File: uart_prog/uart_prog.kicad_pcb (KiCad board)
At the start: 2 copper layers, 22 parts, among them J1 USB_B_Micro, J2 Conn_01x06, Q1 MBT3904DW1, SW1 SW_SPDT, U1 FT231XQ

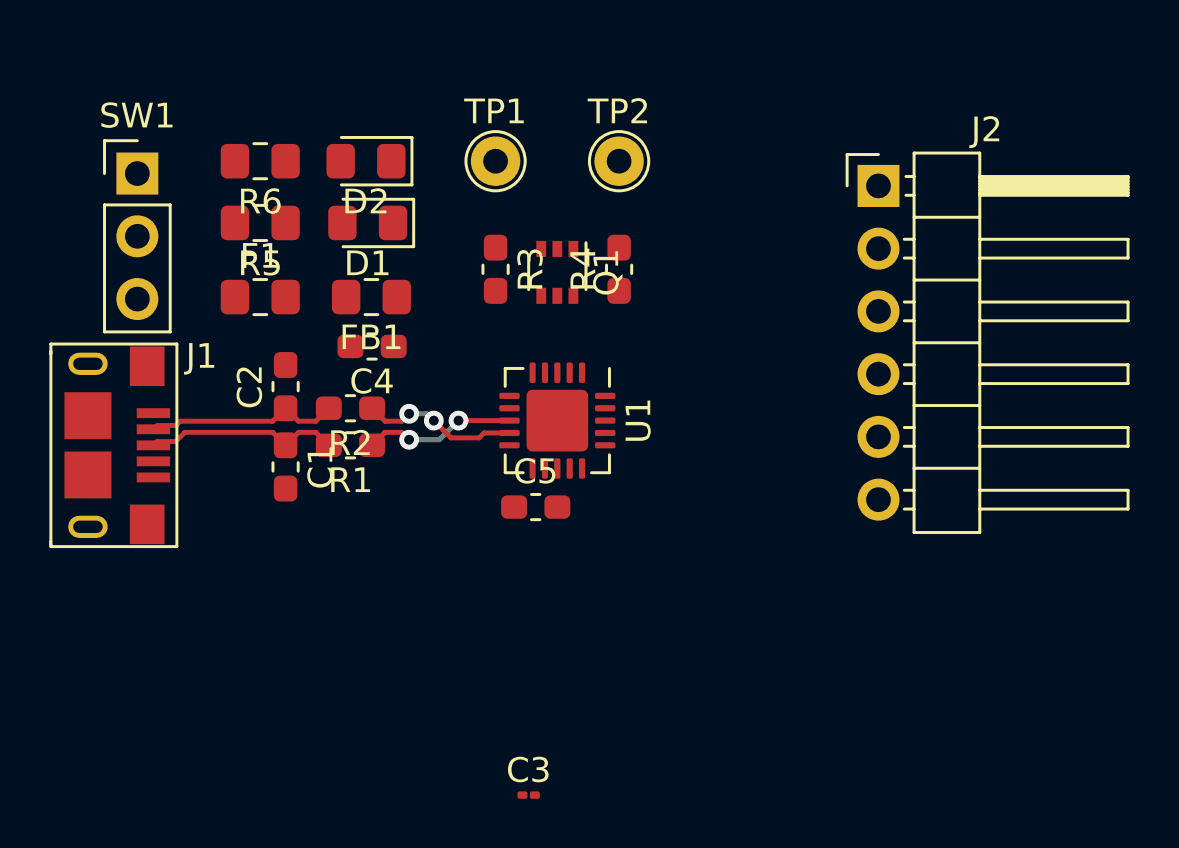
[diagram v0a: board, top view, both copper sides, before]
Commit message: Layout doner
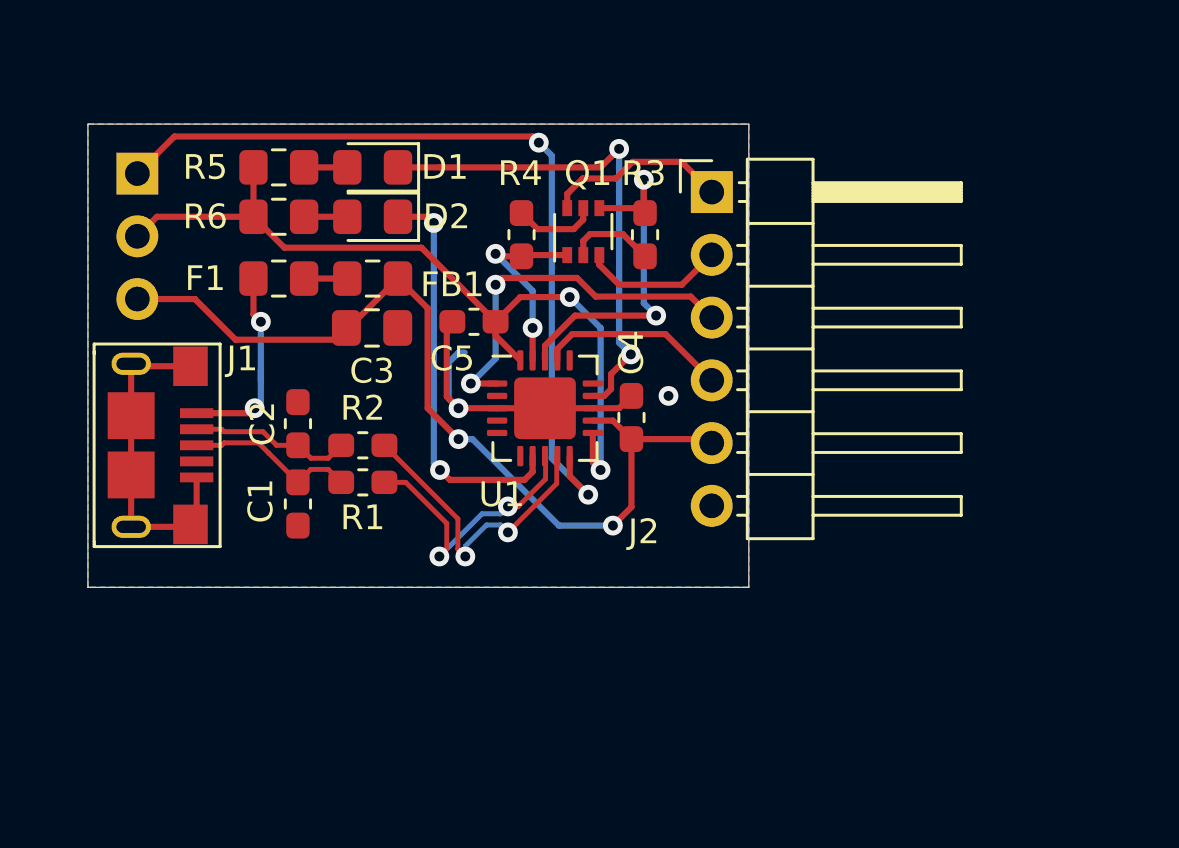
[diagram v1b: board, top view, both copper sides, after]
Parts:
- removed TP1, TP2: TestPoint, TestPoint:TestPoint_THTPad_D2.0mm_Drill1.0mm
- C3: footprint Capacitor_SMD:C_01005_0402Metric -> Capacitor_SMD:C_0805_2012Metric_Pad1.18x1.45mm_HandSolder
- SW1: moved to B.Cu
- moved C3 19.9 mm to (146.5, 84.2)
- moved C4 10.9 mm to (157.0, 87.9), turned to 90 degrees
- moved C5 7.91 mm to (150.6, 84.0), turned to 180 degrees
- moved J2 6.75 mm to (160.2, 78.8)
- moved R3 6.21 mm to (157.6, 80.5), turned to 90 degrees
- moved R4 4.19 mm to (152.6, 80.5), turned to 270 degrees
- moved R5 2.37 mm to (142.7, 77.8)
- moved R6 2.37 mm to (142.7, 79.8)
- moved D2 2.27 mm to (146.5, 79.8)
- moved D1 2.26 mm to (146.5, 77.8)
- moved Q1 1.96 mm to (155.1, 80.3), turned to 90 degrees
- moved J1 1.75 mm to (136.8, 89.0)
- moved C1 1.58 mm to (143.5, 91.4)
- moved C2 1.58 mm to (143.5, 88.1)
- moved R1 1.58 mm to (146.1, 90.5)
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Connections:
- J1 pad 4: (no net) -> Net-(J1-Pad4)
- J2 pad 1: rx -> EN
- J2 pad 2: tx -> BOOT_OPT
- J2 pad 3: EN -> rx
- J2 pad 4: BOOT_OPT -> tx
- U1 pad 15: (no net) -> Net-(U1-Pad15)
- U1 pad 16: (no net) -> Net-(U1-Pad16)
- U1 pad 2: (no net) -> Net-(U1-Pad2)
- U1 pad 4: (no net) -> Net-(U1-Pad4)
- U1 pad 5: (no net) -> Net-(U1-Pad5)
- U1 pad 6: (no net) -> Net-(U1-Pad6)
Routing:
- net 5v: track 0.00 -> 36.5 mm, vias 0 -> 2
- net 3v3: track 0.00 -> 33.9 mm, vias 0 -> 2
- net vccio: track 0.00 -> 33.1 mm, vias 0 -> 2
- net GND: track 0.00 -> 27.3 mm, vias 0 -> 2
- net rxled: track 0.00 -> 20.4 mm, vias 0 -> 2
- net txled: track 0.00 -> 16.3 mm, vias 0 -> 2
- net rx: track 0.00 -> 15.0 mm, vias 0 -> 2
- net dtr: track 0.00 -> 14.6 mm, vias 0 -> 2
- net Net-(F1-Pad1): track 0.00 -> 8.41 mm, vias 0 -> 2
- net rts: track 0.00 -> 7.90 mm, vias 0 -> 2
- net tx: track 0.00 -> 7.73 mm
- net EN: track 0.00 -> 7.47 mm
- net /in2-: track 6.39 -> 12.4 mm
- net BOOT_OPT: track 0.00 -> 5.78 mm
- net /in2+: track 6.23 -> 11.2 mm
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- added copper zone on B.Cu, net GND
- added copper zone on F.Cu, net GND
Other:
- board outline added: 26.8 x 18.8 mm

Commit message: Pcb rev1
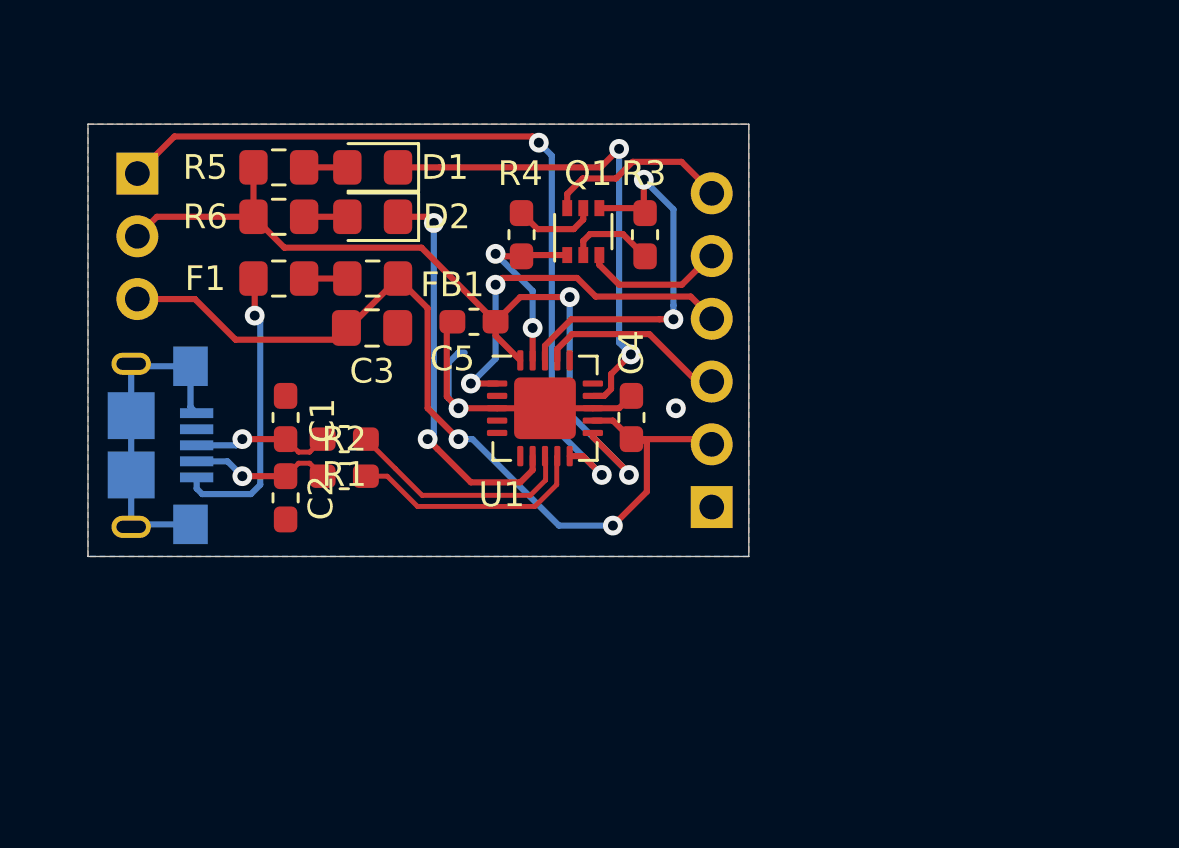
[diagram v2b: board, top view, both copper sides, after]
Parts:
- J1, J2: moved to B.Cu
- moved J2 12.8 mm to (160.2, 91.5)
- moved C1 3.54 mm to (143.0, 87.9), turned to 90 degrees
- moved C2 3.04 mm to (143.0, 91.1), turned to 270 degrees
- moved R1 1.90 mm to (145.4, 88.8)
- moved R2 1.46 mm to (145.4, 90.2)
- turned J1 to 90 degrees
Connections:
- J1 pad 4: Net-(J1-Pad4) -> (no net)
- J2 pad 1: EN -> GND
- J2 pad 2: BOOT_OPT -> 5v
- J2 pad 3: rx -> tx
- J2 pad 4: tx -> rx
- J2 pad 5: 5v -> BOOT_OPT
- J2 pad 6: GND -> EN
- U1 pad 15: Net-(U1-Pad15) -> (no net)
- U1 pad 16: Net-(U1-Pad16) -> (no net)
- U1 pad 2: Net-(U1-Pad2) -> (no net)
- U1 pad 4: Net-(U1-Pad4) -> (no net)
- U1 pad 5: Net-(U1-Pad5) -> (no net)
- U1 pad 6: Net-(U1-Pad6) -> (no net)
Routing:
- net Net-(F1-Pad1): track 8.41 -> 11.7 mm, vias 2 -> 1
- net /in2-: track 12.4 -> 9.76 mm, vias 2 -> 0
- net /in2+: track 11.2 -> 9.45 mm, vias 2 -> 0
- net vccio: track 33.1 -> 34.5 mm
- net /in+: track 6.99 -> 5.64 mm, vias 0 -> 1
- net dtr: track 14.6 -> 15.7 mm
- net 3v3: track 33.9 -> 33.1 mm
- net 5v: track 36.5 -> 37.3 mm
- net /in-: track 6.55 -> 5.78 mm, vias 0 -> 1
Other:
- board size 26.8 x 18.8 mm -> 26.8 x 17.5 mm
- board text added: "3v3"
- board text added: "5v"
- board text added: "EN BOOT RX TX 5V GND"

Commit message: Add schematic back again ...
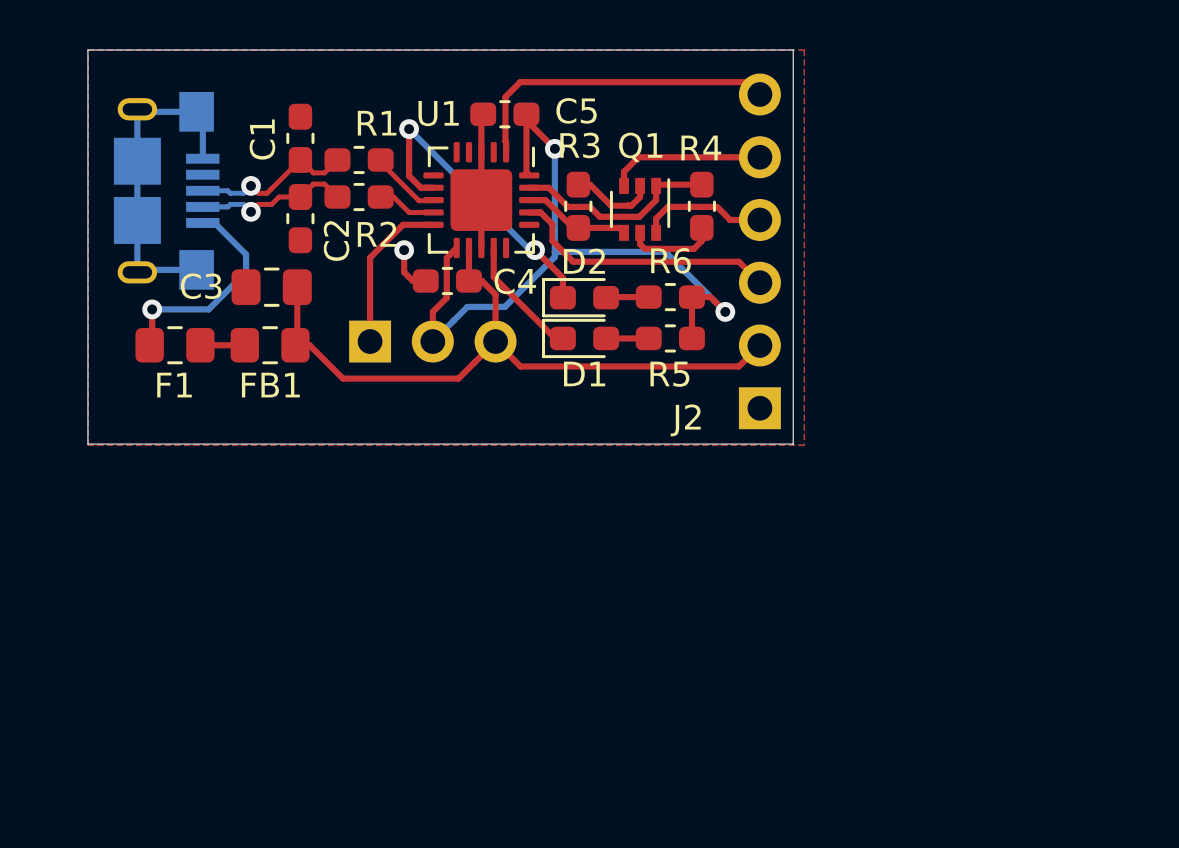
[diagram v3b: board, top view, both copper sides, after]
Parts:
- D1, D2: footprint LED_SMD:LED_0805_2012Metric_Pad1.15x1.40mm_HandSolder -> LED_SMD:LED_0603_1608Metric_Pad1.05x0.95mm_HandSolder
- R5, R6: footprint Resistor_SMD:R_0805_2012Metric_Pad1.15x1.40mm_HandSolder -> Resistor_SMD:R_0603_1608Metric_Pad1.05x0.95mm_HandSolder
- moved R5 17.3 mm to (158.6, 84.7), turned to 0 degrees
- moved R6 16.2 mm to (158.6, 83.0), turned to 0 degrees
- moved SW1 11.6 mm to (146.4, 84.8), turned to 270 degrees
- moved C1 11.3 mm to (143.6, 76.6)
- moved C2 11.3 mm to (143.6, 79.8)
- moved R1 11.3 mm to (146.0, 77.5)
- moved R2 11.3 mm to (146.0, 79.0)
- moved D1 11.0 mm to (155.1, 84.7), turned to 0 degrees
- moved J1 10.3 mm to (137.0, 78.7)
- moved C4 9.28 mm to (149.6, 82.3), turned to 180 degrees
- moved D2 9.18 mm to (155.1, 83.0), turned to 0 degrees
- moved U1 8.81 mm to (150.9, 79.1), turned to 270 degrees
- moved C5 8.49 mm to (151.9, 75.6)
- moved R4 7.39 mm to (159.8, 79.3), turned to 90 degrees
- moved F1 4.99 mm to (138.5, 85.0)
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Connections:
- J2 pad 4: rx -> EN
- J2 pad 6: EN -> rx
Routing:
- net 3v3: track 33.1 -> 6.51 mm, vias 2 -> 0
- net rxled: track 20.4 -> 5.01 mm, vias 2 -> 0
- net dtr: track 15.7 -> 4.39 mm, vias 2 -> 0
- net 5v: track 37.3 -> 27.7 mm, vias 2 -> 0
- net /in2-: track 9.76 -> 2.40 mm
- net /in2+: track 9.45 -> 2.89 mm
- net GND: track 27.3 -> 20.8 mm, vias 2 -> 1
- net vccio: track 34.5 -> 30.5 mm
- net txled: track 16.2 -> 12.6 mm
- net tx: track 7.73 -> 10.9 mm
- net Net-(F1-Pad1): track 11.7 -> 8.91 mm
- net EN: track 7.47 -> 5.19 mm
- net rx: track 15.0 -> 13.0 mm, vias 2 -> 0
- net /in+: track 5.64 -> 6.73 mm
- net BOOT_OPT: track 5.78 -> 6.32 mm
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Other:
- board size 26.8 x 17.5 mm -> 28.6 x 16 mm
- board text added: "RX BOOT EN TX 5v GND"
- board text removed: "EN BOOT RX TX 5V GND"
